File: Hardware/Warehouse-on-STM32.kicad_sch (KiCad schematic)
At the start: 16 parts, among them SW1 SW_DPST, SW2 SW_DPST, SW3 SW_DPST, SW4 SW_DPST, U1 STM32F103C8Tx, Y2 Crystal

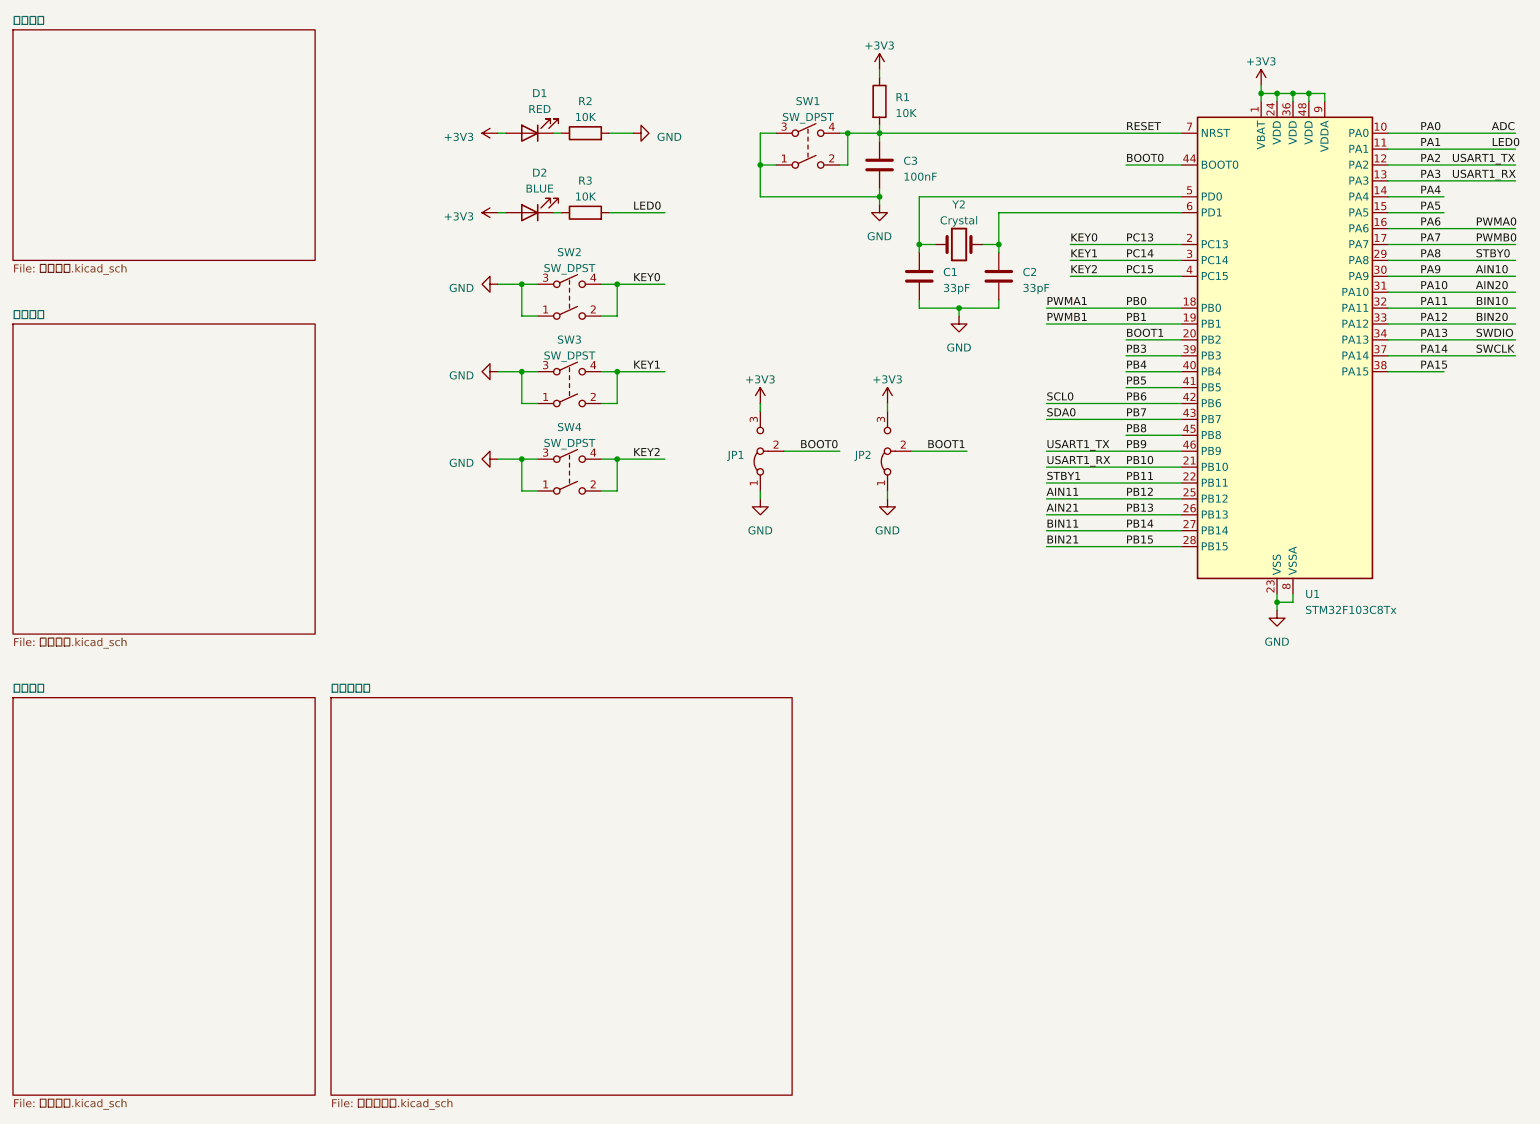
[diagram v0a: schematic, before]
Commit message: 2023/3/29
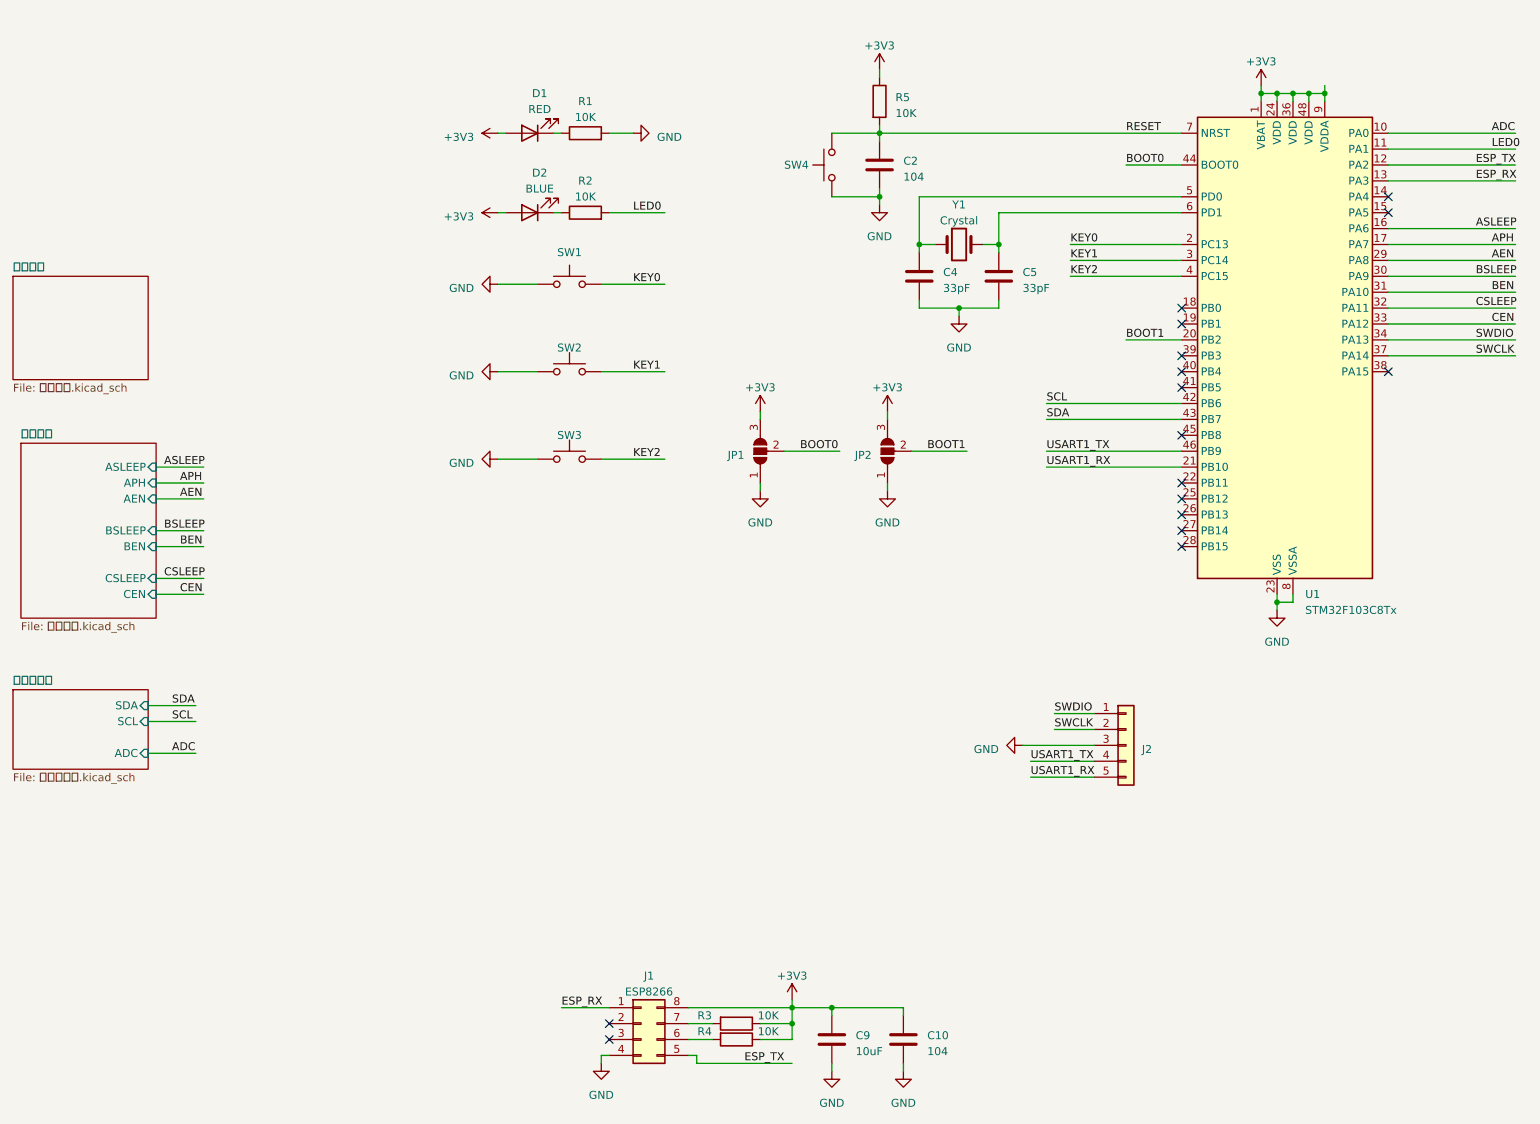
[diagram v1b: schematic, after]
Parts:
- removed JP1, JP2: Jumper_3_Bridged12, symbol Jumper:Jumper_3_Bridged12
- removed SW1, SW2, SW3, SW4: SW_DPST, symbol Switch:SW_DPST
- added C10: 104, Capacitor_SMD:C_0402_1005Metric, symbol Device:C
- added C9: 10uF, Capacitor_SMD:C_0603_1608Metric, symbol Device:C
- added J1: ESP8266, Connector_PinSocket_2.54mm:PinSocket_2x04_P2.54mm_Vertical, symbol Connector_Generic:Conn_02x04_Counter_Clockwise
- added J2: Conn_01x05, Connector_PinHeader_2.54mm:PinHeader_1x05_P2.54mm_Vertical, symbol Connector_Generic:Conn_01x05
- added JP1, JP2: SolderJumper_3_Open, Jumper:SolderJumper-3_P2.0mm_Open_TrianglePad1.0x1.5mm, symbol Jumper:SolderJumper_3_Open
- added R3, R4: 10K, Resistor_SMD:R_0402_1005Metric, symbol Device:R
- added SW1, SW2, SW3, SW4: SW_Push, Button_Switch_SMD:SW_Tactile_SPST_NO_Straight_CK_PTS636Sx25SMTRLFS, symbol Switch:SW_Push
- C2: renamed from C3; value 100nF -> 104; footprint (none) -> Capacitor_SMD:C_0402_1005Metric
- C4: renamed from C1; footprint (none) -> Capacitor_SMD:C_0402_1005Metric
- C5: renamed from C2; footprint (none) -> Capacitor_SMD:C_0402_1005Metric
- D1, D2: footprint (none) -> LED_SMD:LED_0402_1005Metric
- R1: renamed from R2; footprint (none) -> Resistor_SMD:R_0402_1005Metric
- R2: renamed from R3; footprint (none) -> Resistor_SMD:R_0402_1005Metric
- R5: renamed from R1; footprint (none) -> Resistor_SMD:R_0402_1005Metric
- renumbered Y2 to Y1
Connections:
- net +3V3: now also C10.1, C9.1, J1.8 (Pin_8), JP1.3 (B), JP2.3 (B), R3.1, R4.1
- net BOOT0: now also JP1.2 (C)
- net BOOT1: now also JP2.2 (C)
- net GND: now also C10.2, C9.2, J1.4 (Pin_4), J2.3 (Pin_3), JP1.1 (A), JP2.1 (A), SW1.1, SW2.1, SW3.1, SW4.1
- net KEY0: now also SW1.2
- net KEY1: now also SW2.2
- net KEY2: now also SW3.2
- net RESET: now also SW4.2
- net AIN10 renamed BSLEEP
- net AIN11: no longer names the net of U1.25 (PB12)
- net AIN20 renamed BEN
- net AIN21: no longer names the net of U1.26 (PB13)
- net BIN10 renamed CSLEEP
- net BIN11: no longer names the net of U1.27 (PB14)
- net BIN20 renamed CEN
- net BIN21: no longer names the net of U1.28 (PB15)
- net PA13 renamed SWDIO
- net SWDIO: now also J2.1 (Pin_1)
- net PA14 renamed SWCLK
- net SWCLK: now also J2.2 (Pin_2)
- net PA15: no longer names the net of U1.38 (PA15)
- net PA2 renamed ESP_TX
- net ESP_TX: now also J1.5 (Pin_5); no longer U1.46 (PB9)
- net PA3 renamed ESP_RX
- net ESP_RX: now also J1.1 (Pin_1); no longer U1.21 (PB10)
- net PA4: no longer names the net of U1.14 (PA4)
- net PA5: no longer names the net of U1.15 (PA5)
- net PA6 renamed ASLEEP
- net PA7 renamed APH
- net PA8 renamed AEN
- net PB0: no longer names the net of U1.18 (PB0)
- net PB1: no longer names the net of U1.19 (PB1)
- net PB11: no longer names the net of U1.22 (PB11)
- net PB3: no longer names the net of U1.39 (PB3)
- net PB4: no longer names the net of U1.40 (PB4)
- net PB5: no longer names the net of U1.41 (PB5)
- net PB6 renamed SCL
- net PB7 renamed SDA
- net PB8: no longer names the net of U1.45 (PB8)
- new net: J1.6 (Pin_6), R4.2
- new net: J1.7 (Pin_7), R3.2
- new net USART1_RX: J2.5 (Pin_5), U1.21 (PB10)
- new net USART1_TX: J2.4 (Pin_4), U1.46 (PB9)
- no-connect marks 0 -> 16
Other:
- removed sheet 通信模块
- sheet 传感器模块 ports: added ADC, SCL, SDA; removed none
- sheet 驱动模块 ports: added AEN, APH, ASLEEP, BEN, BSLEEP, CEN, CSLEEP; removed none
